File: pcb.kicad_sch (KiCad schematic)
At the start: 21 parts, among them U1 Pico

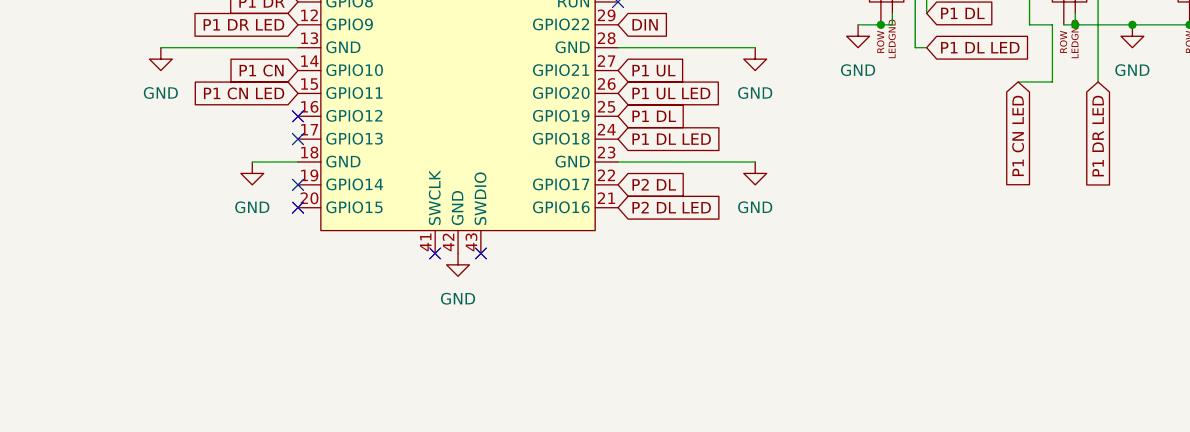
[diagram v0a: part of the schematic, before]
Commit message: add test/service buttons (oops)
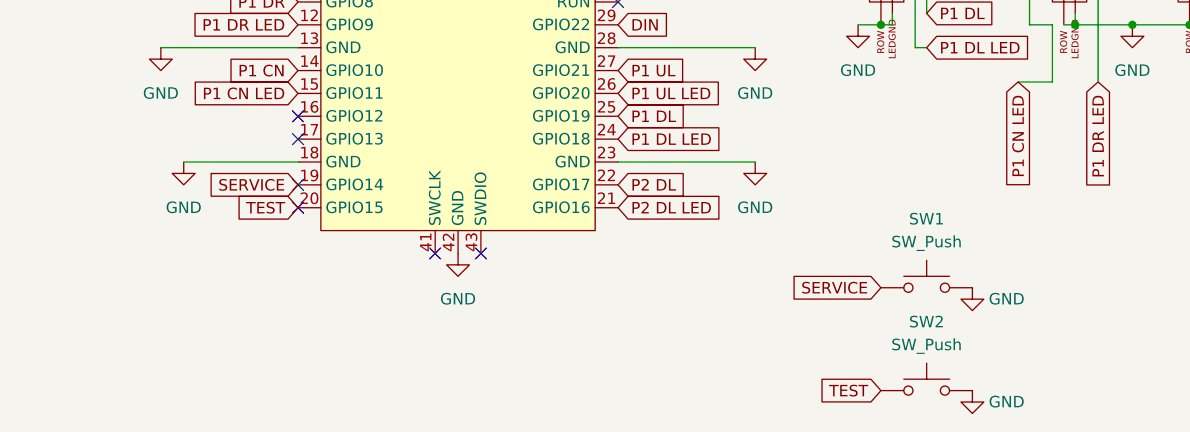
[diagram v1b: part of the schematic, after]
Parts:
- added SW1, SW2: SW_Push, Button_Switch_THT:SW_PUSH_6mm, symbol Switch:SW_Push
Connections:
- net GND: now also SW1.2, SW2.2
- net SERVICE: now reaches U1.19 (GPIO14)
- net SERVICE: now also SW1.1
- net TEST: now reaches U1.20 (GPIO15)
- net TEST: now also SW2.1
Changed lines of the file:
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@@
     (stroke (width 0) (type default) (color 0 0 0 0))
   )
-  (wire (pts (xy 121.92 118.11) (xy 127 118.11))
+  (wire (pts (xy 114.3 118.11) (xy 127 118.11))
     (stroke (width 0) (type default) (color 0 0 0 0))
   )
@@
     )
   )
+  (global_label "TEST" (shape input) (at 127 123.19 180) (fields_autoplaced)
+    (effects (font (size 1.27 1.27)) (justify right))
+    (property "Intersheet References" "${INTERSHEET_REFS}" (id 0) (at 120.2931 123.1106 0)
+      (effects (font (size 1.27 1.27)) (justify right) hide)
+    )
+  )
   (global_label "P2 UL" (shape input) (at 232.41 73.66 0) (fields_autoplaced)
     (effects (font (size 1.27 1.27)) (justify left))
@@
     )
   )
+  (global_label "SERVICE" (shape input) (at 127 120.65 180) (fields_autoplaced)
+    (effects (font (size 1.27 1.27)) (justify right))
+    (property "Intersheet References" "${INTERSHEET_REFS}" (id 0) (at 116.8459 120.5706 0)
+      (effects (font (size 1.27 1.27)) (justify right) hide)
+    )
+  )
   (global_label "P2 CN LED" (shape input) (at 127 85.09 180) (fields_autoplaced)
     (effects (font (size 1.27 1.27)) (justify right))
@@
     )
   )
+  (global_label "SERVICE" (shape input) (at 191.77 132.08 180) (fields_autoplaced)
+    (effects (font (size 1.27 1.27)) (justify right))
+    (property "Intersheet References" "${INTERSHEET_REFS}" (id 0) (at 181.6159 132.0006 0)
+      (effects (font (size 1.27 1.27)) (justify right) hide)
+    )
+  )
   (global_label "P1 UR" (shape input) (at 127 95.25 180) (fields_autoplaced)
     (effects (font (size 1.27 1.27)) (justify right))
@@
     )
   )
+  (global_label "TEST" (shape input) (at 191.77 143.51 180) (fields_autoplaced)
+    (effects (font (size 1.27 1.27)) (justify right))
+    (property "Intersheet References" "${INTERSHEET_REFS}" (id 0) (at 185.0631 143.4306 0)
+      (effects (font (size 1.27 1.27)) (justify right) hide)
+    )
+  )
   (global_label "P2 DR" (shape input) (at 127 87.63 180) (fields_autoplaced)
     (effects (font (size 1.27 1.27)) (justify right))
@@
     )
   )
-  (symbol (lib_id "power:GND") (at 121.92 118.11 0) (unit 1)
-    (in_bom yes) (on_board yes) (fields_autoplaced)
-    (property "Reference" "#PWR0108" (id 0) (at 121.92 124.46 0)
-      (effects (font (size 1.27 1.27)) hide)
-    )
-    (property "Value" "GND" (id 1) (at 121.92 123.19 0))
-    (property "Footprint" "" (id 2) (at 121.92 118.11 0)
-      (effects (font (size 1.27 1.27)) hide)
-    )
-    (property "Datasheet" "" (id 3) (at 121.92 118.11 0)
+  (symbol (lib_id "Switch:SW_Push") (at 196.85 132.08 0) (unit 1)
+    (in_bom yes) (on_board yes) (fields_autoplaced)
+    (property "Reference" "SW1" (id 0) (at 196.85 124.46 0))
+    (property "Value" "SW_Push" (id 1) (at 196.85 127 0))
+    (property "Footprint" "Button_Switch_THT:SW_PUSH_6mm" (id 2) (at 196.85 127 0)
+      (effects (font (size 1.27 1.27)) hide)
+    )
+    (property "Datasheet" "~" (id 3) (at 196.85 127 0)
+      (effects (font (size 1.27 1.27)) hide)
+    )
+    (pin "1")
+    (pin "2")
+  )
+  (symbol (lib_id "power:GND") (at 114.3 118.11 0) (unit 1)
+    (in_bom yes) (on_board yes) (fields_autoplaced)
+    (property "Reference" "#PWR0108" (id 0) (at 114.3 124.46 0)
+      (effects (font (size 1.27 1.27)) hide)
+    )
+    (property "Value" "GND" (id 1) (at 114.3 123.19 0))
+    (property "Footprint" "" (id 2) (at 114.3 118.11 0)
+      (effects (font (size 1.27 1.27)) hide)
+    )
+    (property "Datasheet" "" (id 3) (at 114.3 118.11 0)
       (effects (font (size 1.27 1.27)) hide)
     )
@@
     )
     (pin "1")
+  )
+  (symbol (lib_id "Switch:SW_Push") (at 196.85 143.51 0) (unit 1)
+    (in_bom yes) (on_board yes) (fields_autoplaced)
+    (property "Reference" "SW2" (id 0) (at 196.85 135.89 0))
+    (property "Value" "SW_Push" (id 1) (at 196.85 138.43 0))
+    (property "Footprint" "Button_Switch_THT:SW_PUSH_6mm" (id 2) (at 196.85 138.43 0)
+      (effects (font (size 1.27 1.27)) hide)
+    )
+    (property "Datasheet" "~" (id 3) (at 196.85 138.43 0)
+      (effects (font (size 1.27 1.27)) hide)
+    )
+    (pin "1")
+    (pin "2")
   )
   (symbol (lib_id "LED:WS2812B") (at 198.12 50.8 180) (unit 1)
@@
     (pin "1")
   )
+  (symbol (lib_id "power:GND") (at 201.93 132.08 0) (unit 1)
+    (in_bom yes) (on_board yes)
+    (property "Reference" "#PWR01" (id 0) (at 201.93 138.43 0)
+      (effects (font (size 1.27 1.27)) hide)
+    )
+    (property "Value" "GND" (id 1) (at 205.74 133.35 0))
+    (property "Footprint" "" (id 2) (at 201.93 132.08 0)
+      (effects (font (size 1.27 1.27)) hide)
+    )
+    (property "Datasheet" "" (id 3) (at 201.93 132.08 0)
+      (effects (font (size 1.27 1.27)) hide)
+    )
+    (pin "1")
+  )
   (symbol (lib_id "power:GND") (at 240.03 92.71 0) (unit 1)
     (in_bom yes) (on_board yes) (fields_autoplaced)
@@
     (pin "3")
     (pin "4")
+  )
+  (symbol (lib_id "power:GND") (at 201.93 143.51 0) (unit 1)
+    (in_bom yes) (on_board yes)
+    (property "Reference" "#PWR02" (id 0) (at 201.93 149.86 0)
+      (effects (font (size 1.27 1.27)) hide)
+    )
+    (property "Value" "GND" (id 1) (at 205.74 144.78 0))
+    (property "Footprint" "" (id 2) (at 201.93 143.51 0)
+      (effects (font (size 1.27 1.27)) hide)
+    )
+    (property "Datasheet" "" (id 3) (at 201.93 143.51 0)
+      (effects (font (size 1.27 1.27)) hide)
+    )
+    (pin "1")
   )
   (symbol (lib_id "power:GND") (at 144.78 128.27 0) (unit 1)
@@
       (reference "#FLG0101") (unit 1) (value "PWR_FLAG") (footprint "")
     )
+    (path "/c9028cf3-78dd-4027-9d7b-6c668c7d0c91"
+      (reference "#PWR01") (unit 1) (value "GND") (footprint "")
+    )
+    (path "/f2065da4-e15e-4779-9b65-8eb1e0838f97"
+      (reference "#PWR02") (unit 1) (value "GND") (footprint "")
+    )
     (path "/ff704a90-239d-4023-bb2d-df3c8df3a6ac"
       (reference "#PWR0101") (unit 1) (value "GND") (footprint "")
@@
       (reference "MX10") (unit 1) (value "MX-LED") (footprint "MX_Only:MXOnly-1U")
     )
+    (path "/04a1a727-9f82-4149-abb6-b153d2ea070f"
+      (reference "SW1") (unit 1) (value "SW_Push") (footprint "Button_Switch_THT:SW_PUSH_6mm")
+    )
+    (path "/4097679c-fee5-4ca9-b45c-02466706712e"
+      (reference "SW2") (unit 1) (value "SW_Push") (footprint "Button_Switch_THT:SW_PUSH_6mm")
+    )
     (path "/430d1463-de71-4131-a362-3f573ce8f2df"

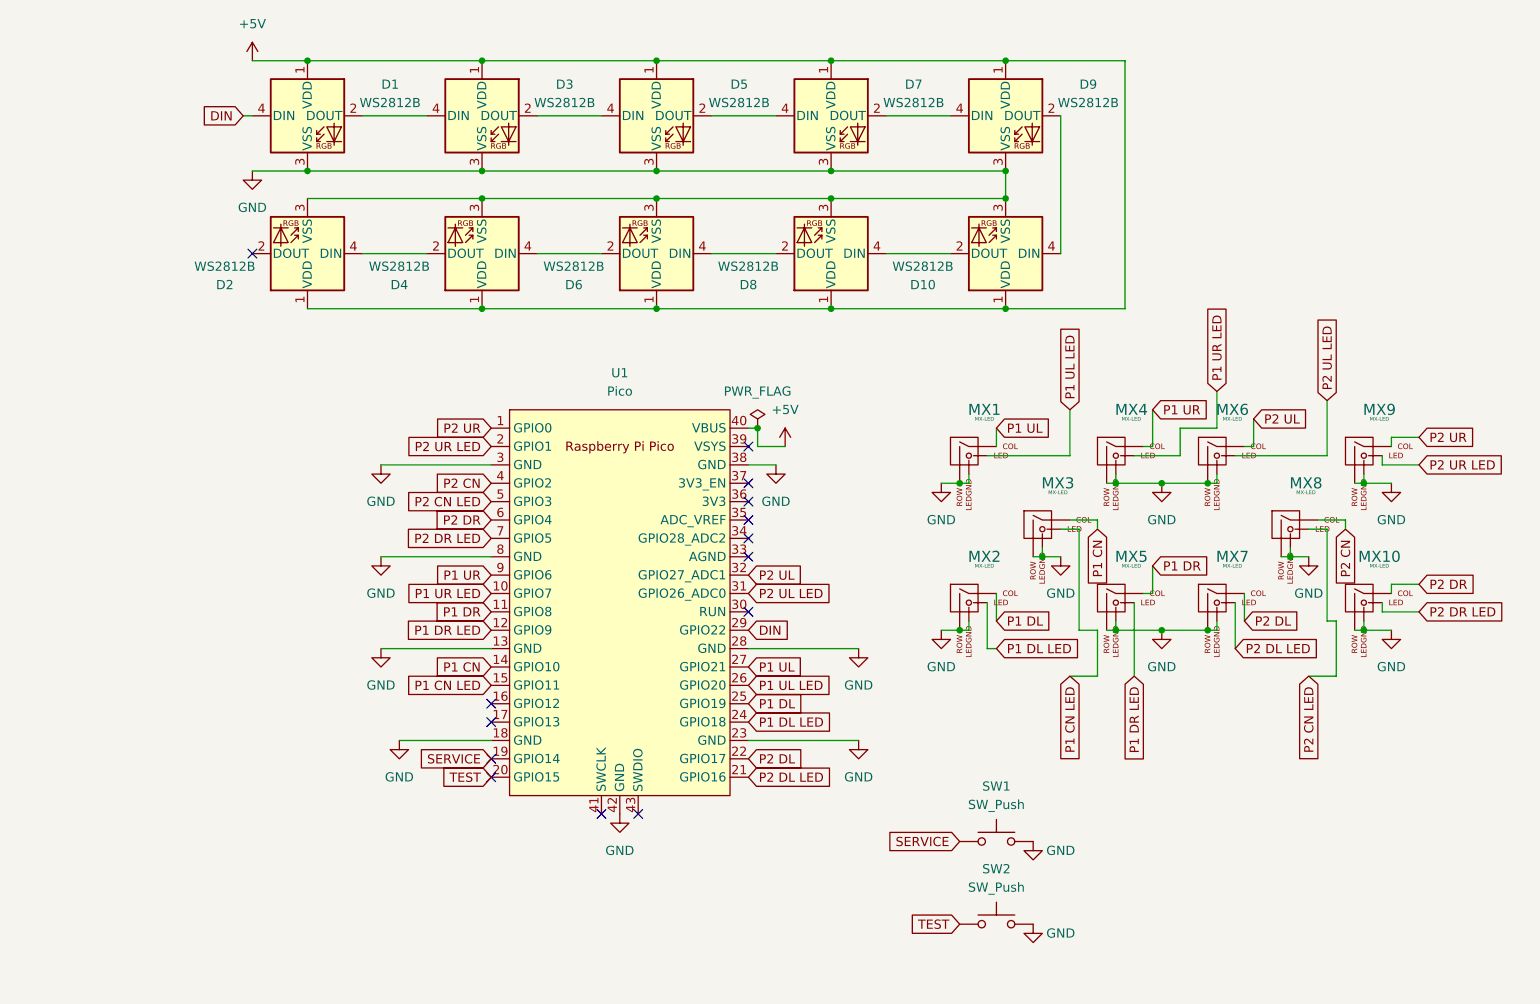
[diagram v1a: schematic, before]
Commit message: Tidy up schematic more
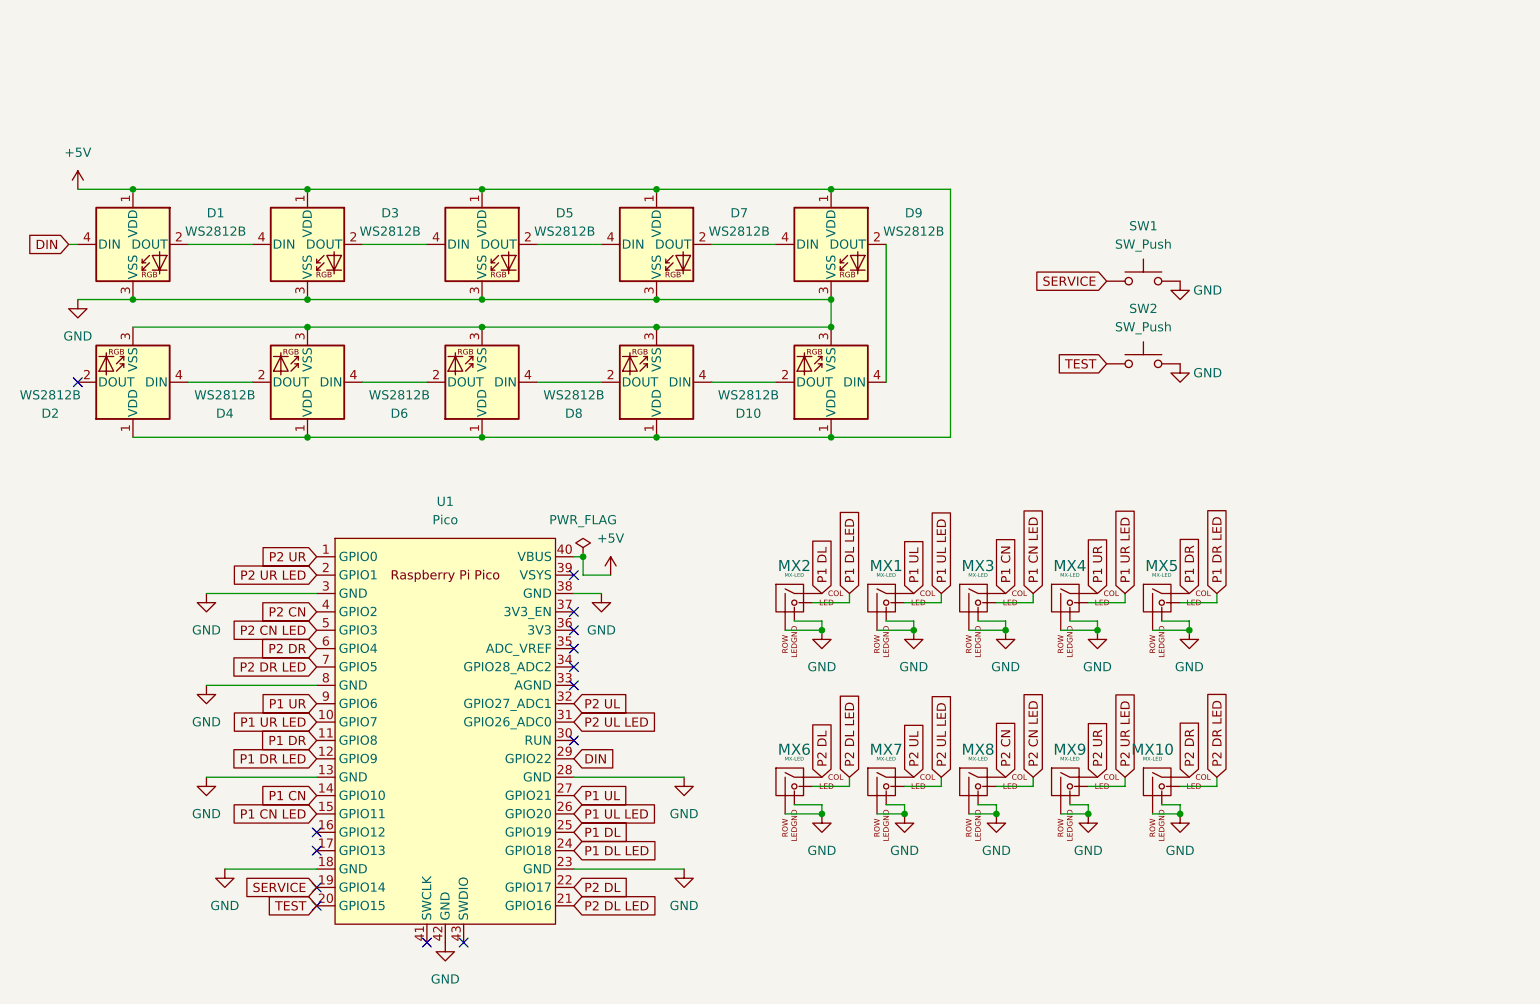
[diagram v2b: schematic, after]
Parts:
- renumbered MX7 to MX6, MX6 to MX7
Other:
- moved on the sheet: D1, D10, D2, D3, D4, D5, D6, D7, D8, D9, MX1, MX10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
